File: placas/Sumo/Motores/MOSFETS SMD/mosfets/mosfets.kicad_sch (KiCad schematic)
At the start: 15 parts, among them J1 Screw_Terminal_01x02, J3 Screw_Terminal_01x02, J5 Conn_01x06_Pin, Q1 IRLZ44N, Q2 IRLZ44N, Q3 IRLZ44N, Q4 IRLZ44N, Q5 IRLZ44N, U1 HIP4082xP

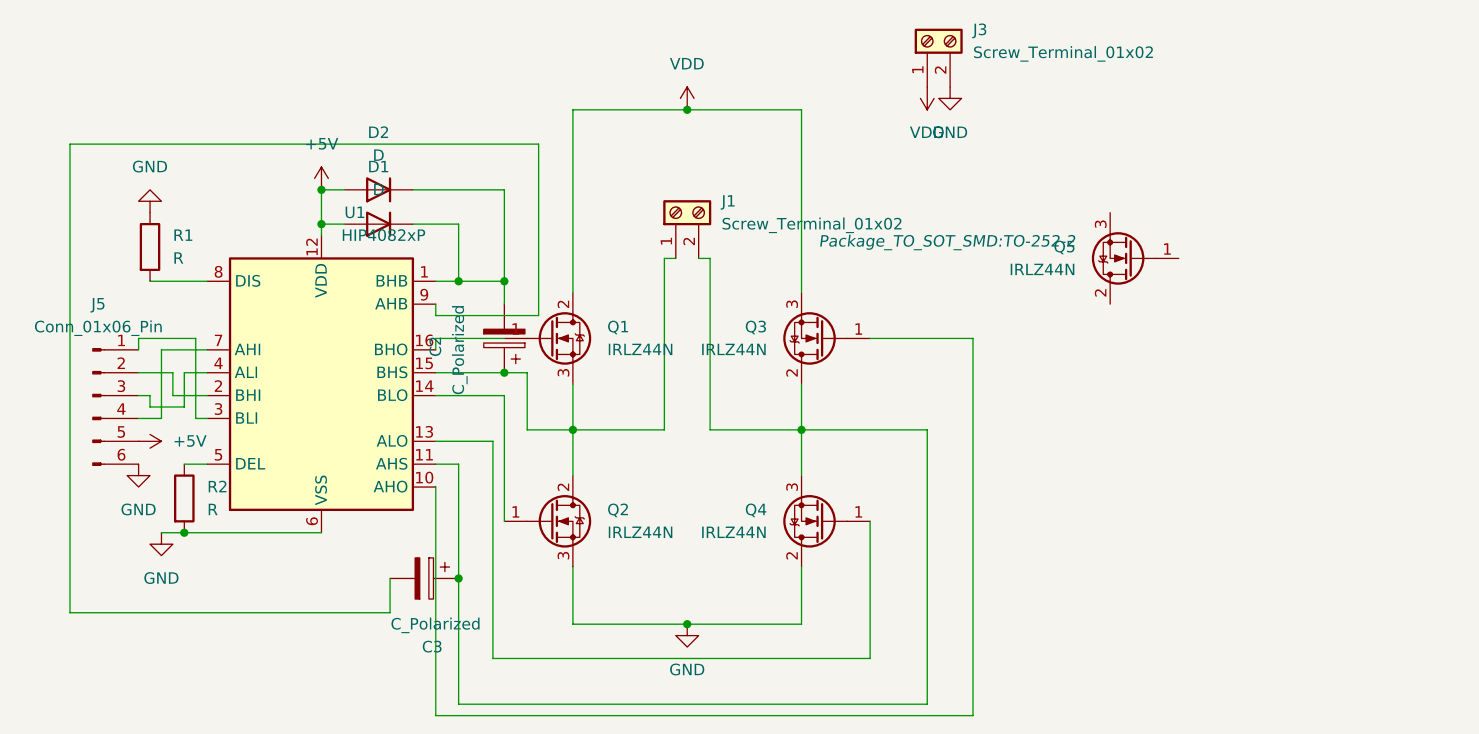
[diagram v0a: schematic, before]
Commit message: dfg
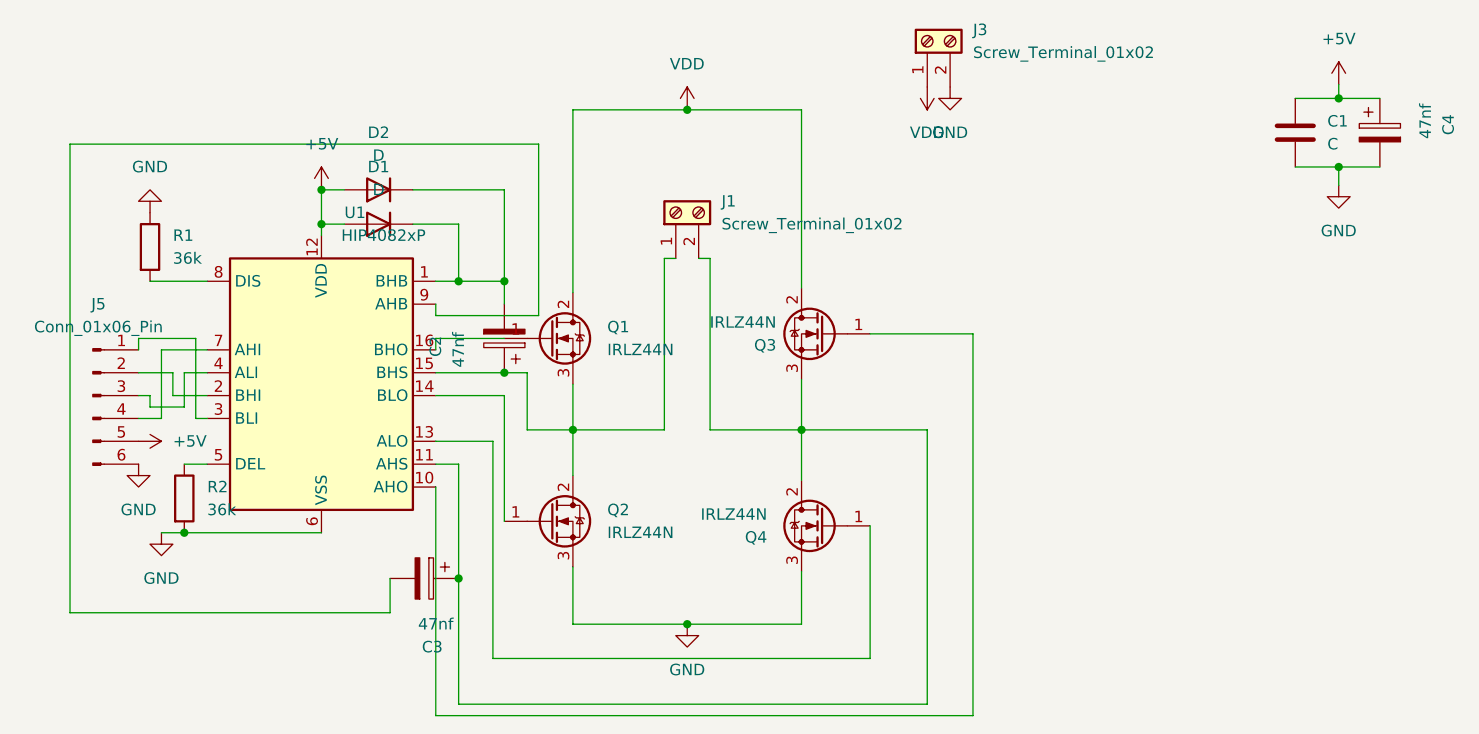
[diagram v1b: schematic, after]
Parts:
- removed Q5: IRLZ44N, Package_TO_SOT_SMD:TO-252-2, symbol Transistor_FET:IRLZ44N
- added C1: C, Capacitor_THT:C_Axial_L5.1mm_D3.1mm_P10.00mm_Horizontal, symbol Device:C
- added C4: 47nf, Capacitor_THT:CP_Radial_D8.0mm_P3.80mm, symbol Device:C_Polarized
- C2, C3: value C_Polarized -> 47nf
- D1, D2: footprint Diode_SMD:D_SOD-123 -> Diode_THT:D_DO-15_P15.24mm_Horizontal
- Q1, Q2, Q3, Q4: footprint Package_TO_SOT_SMD:TO-252-2 -> Package_TO_SOT_THT:TO-220-3_Vertical
- R1, R2: value R -> 36k; footprint Resistor_SMD:R_1206_3216Metric -> Resistor_THT:R_Axial_DIN0309_L9.0mm_D3.2mm_P12.70mm_Horizontal
- U1: footprint Package_SO:SOIC-16_3.9x9.9mm_P1.27mm -> Package_DIP:DIP-16_W7.62mm
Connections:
- net +5V: now also C1.1, C4.1
- net GND: now also Q4.3 (S), C1.2, C4.2; no longer Q4.2 (D)
- net VDD: now also Q3.2 (D); no longer Q3.3 (S)
- net at C3.1, J1.2 (Pin_2), U1.11 (AHS): now also Q3.3 (S), Q4.2 (D); no longer Q3.2 (D), Q4.3 (S)
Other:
- moved on the sheet: Q3, Q4
